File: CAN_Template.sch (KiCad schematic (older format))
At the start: 24 parts, among them U5 MCP2515-xSO, U6 SN65HVD1050D, U7 TXB0104PWR

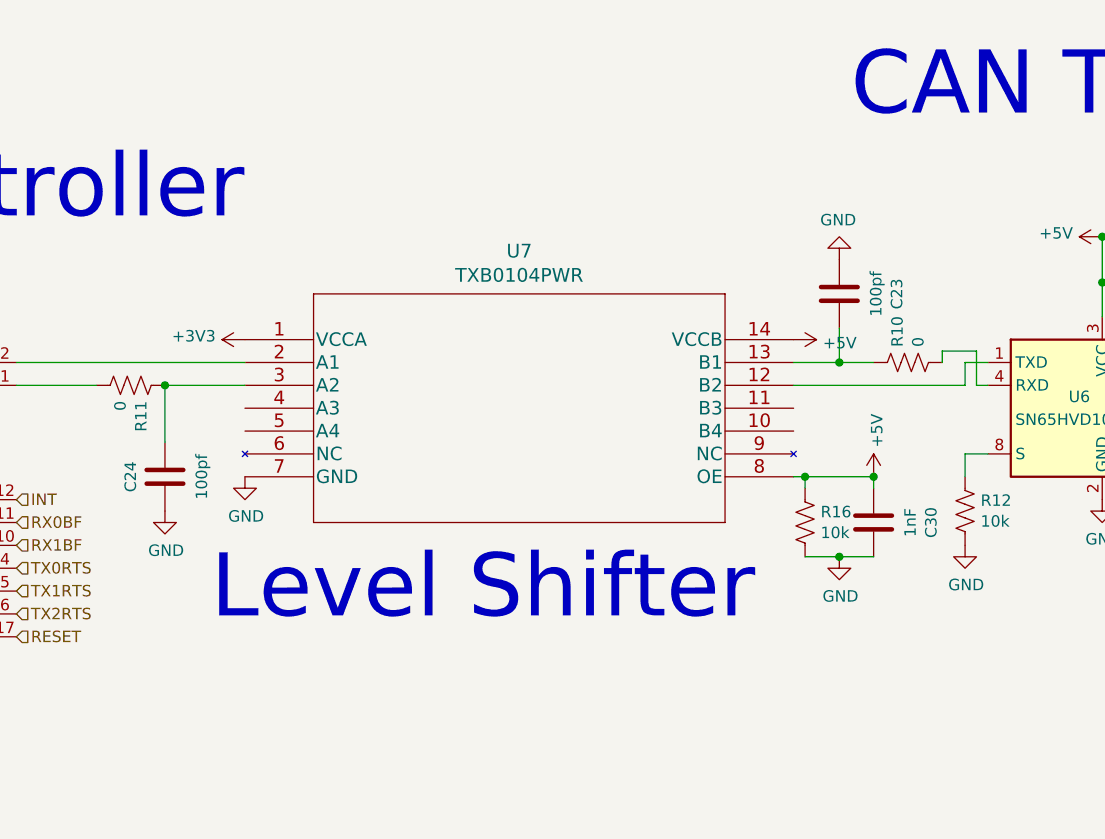
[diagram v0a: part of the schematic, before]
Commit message: Added some filters and stuff
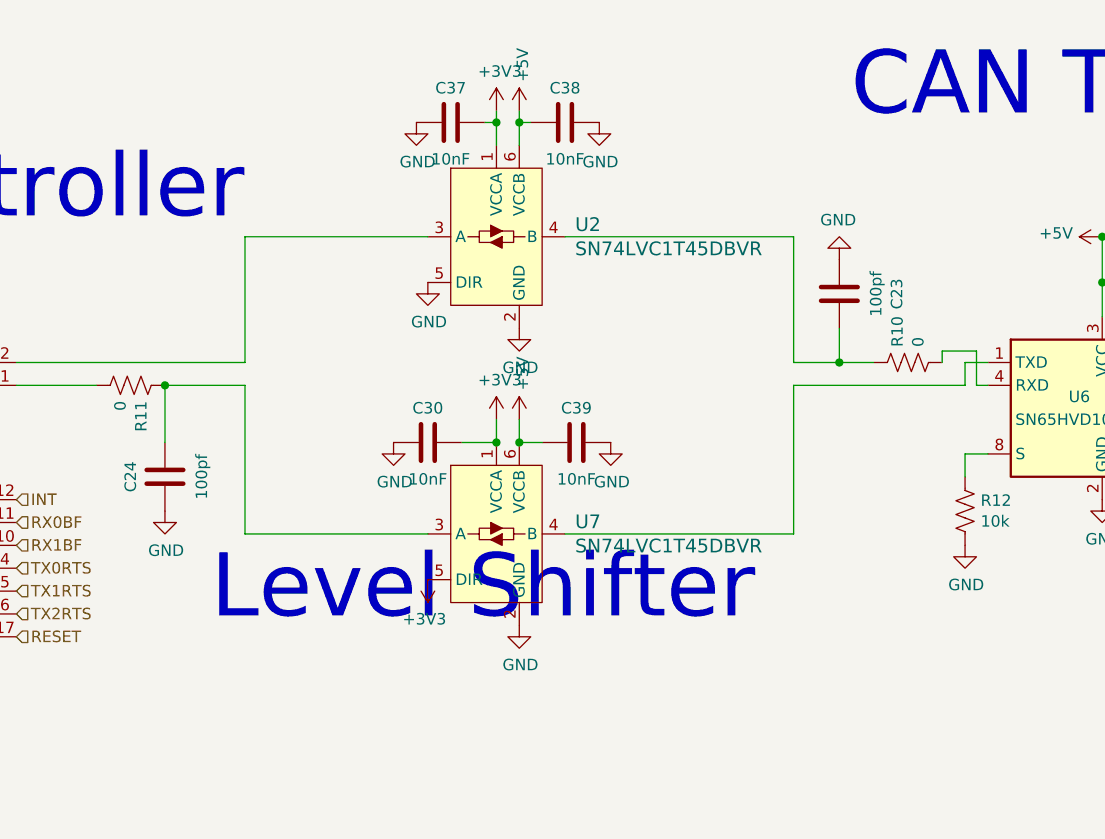
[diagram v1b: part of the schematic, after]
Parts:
- removed R16: 10k, Resistor_SMD:R_0402_1005Metric, symbol Device:R_US
- removed U7: TXB0104PWR, Level Shifter:TXB0104PWR, symbol 2019-12-30_17-25-07:TXB0104PWR
- added C37, C38, C39: 10nF, Capacitor_SMD:C_0402_1005Metric, symbol Device:C
- added U2, U7: SN74LVC1T45DBVR, digikey-footprints:SOT-23-6, symbol dk_Logic-Translators-Level-Shifters:SN74LVC1T45DBVR
- C30: value 1nF -> 10nF
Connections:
- net +3V3: now also C30.2, C37.2, U2.1 (VCCA), U7.1 (VCCA), U7.5 (DIR)
- net +5V: now also C38.1, C39.1, U2.6 (VCCB), U7.6 (VCCB); no longer C30.2
- net GND: now also C37.1, C38.2, C39.2, U2.2 (GND), U2.5 (DIR), U7.2 (GND)
- net at U5.2 (RXCAN): now also U2.3 (A)
- net at C23.1, R10.1: now also U2.4 (B)
- net at U6.1 (TXD): now also U7.4 (B)
- net at C24.2, R11.1: now also U7.3 (A)
